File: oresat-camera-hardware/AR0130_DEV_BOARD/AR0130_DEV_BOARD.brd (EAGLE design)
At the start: 40 x 44 mm, 70 parts, among them J2 4-1734592-0, U10 SN74AVCB164245VR, U11 KC2520B27.0000C10E00, U12 TPS71818-33DRVT, U13 SN74AVCH8T245RHLR, U14 TPS71928-28DRVT, U15 TPS71928-28DRVT, U6 MCP9808T-E/MCDFN8_2X3MC-M, U7 MCP9808T-E/MCDFN8_2X3MC-M, U9 TCA9509DGKRDGK8-M

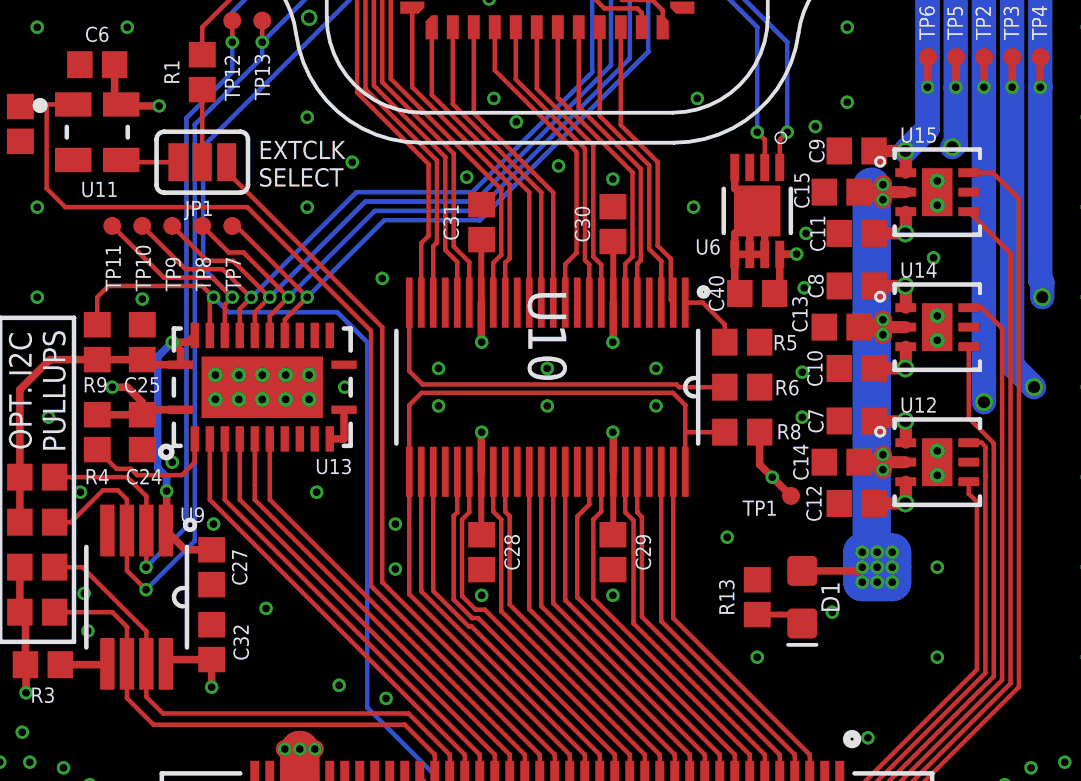
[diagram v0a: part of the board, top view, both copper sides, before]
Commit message: yada yada yada
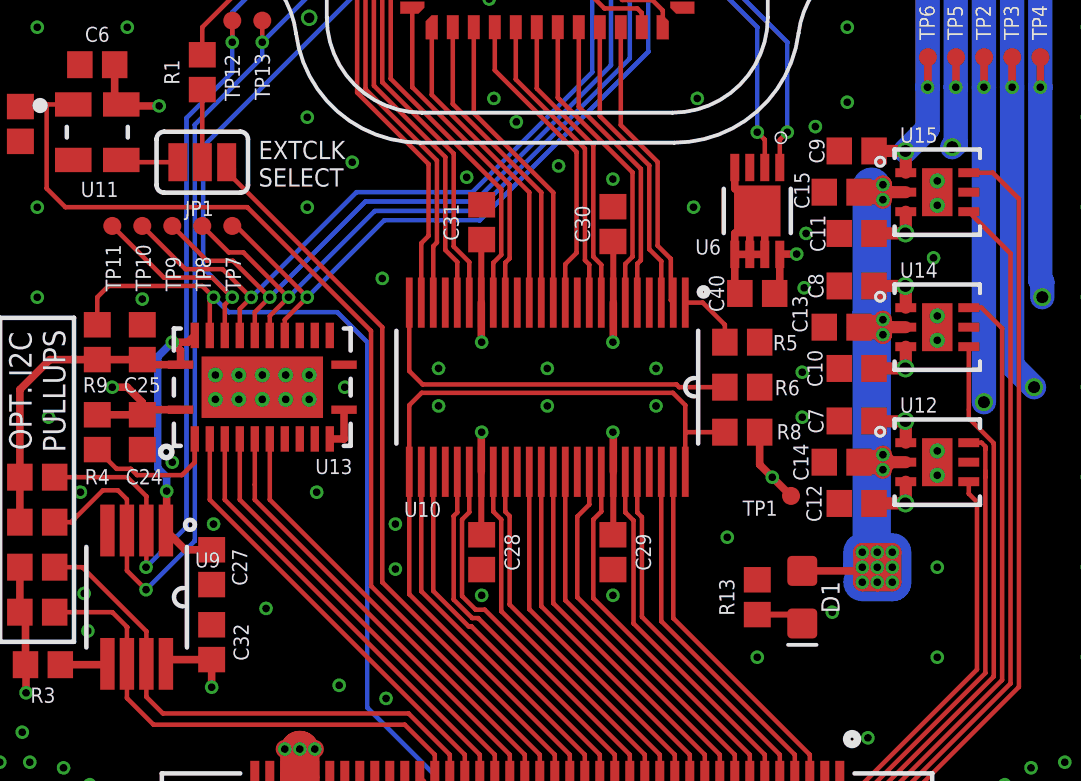
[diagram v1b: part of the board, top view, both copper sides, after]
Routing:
- net 5V: track 65.4 -> 70.4 mm
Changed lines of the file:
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@@
 <element name="U9" library="Oliver_Custom" package="DGK8-M" value="TCA9509DGKRDGK8-M" x="6.3125" y="11" smashed="yes" rot="R270">
 <attribute name="MANUFACTURER_PART_NUMBER" value="TCA9509DGKR" x="6.3125" y="11" size="1.778" layer="27" rot="R270" display="off"/>
-<attribute name="NAME" x="7.7574" y="13.4915" size="0.5" layer="25" font="vector" ratio="15" rot="SR0"/>
+<attribute name="NAME" x="8.2574" y="11.9915" size="0.5" layer="25" font="vector" ratio="15" rot="SR0"/>
 <attribute name="VENDOR" value="Texas Instruments" x="6.3125" y="11" size="1.778" layer="27" rot="R270" display="off"/>
 </element>
 <element name="U10" library="Oliver_Custom" package="DGV48" value="SN74AVCB164245VR" x="20" y="18" smashed="yes" rot="R270">
 <attribute name="MANUFACTURER_PART_NUMBER" value="SN74AVCB164245VR" x="20" y="18" size="1.778" layer="27" rot="R270" display="off"/>
-<attribute name="NAME" x="19.365" y="21.2766" size="1.27" layer="25" ratio="6" rot="SR270"/>
+<attribute name="NAME" x="15.2234" y="13.6775" size="0.5" layer="25" font="vector" ratio="15" rot="SR0"/>
 <attribute name="VENDOR" value="Texas Instruments" x="20" y="18" size="1.778" layer="27" rot="R270" display="off"/>
 </element>
@@
 <wire x1="30.5" y1="12" x2="31.5" y2="12" width="1.27" layer="16"/>
 <wire x1="30.5" y1="12" x2="30.5" y2="12.5" width="1.27" layer="16"/>
-<wire x1="30.5" y1="12.5" x2="30.5" y2="11.5" width="1.27" layer="16"/>
 <wire x1="31.5" y1="11.5" x2="31.5" y2="12.5" width="1.27" layer="16"/>
 <wire x1="30.5" y1="11.5" x2="31.5" y2="11.5" width="1.27" layer="16"/>
@@
 <wire x1="31.1875" y1="15.75" x2="31.1875" y2="15.5" width="0.508" layer="1"/>
 <wire x1="31.1875" y1="15.5" x2="31.1875" y2="15.25" width="0.508" layer="1"/>
-<wire x1="30.3925" y1="15.5" x2="31.1875" y2="15.5" width="0.6096" layer="1"/>
+<wire x1="30.3925" y1="15.5" x2="31.1875" y2="15.5" width="0.8128" layer="1"/>
 <wire x1="31.1875" y1="15.5" x2="31.95" y2="15.5" width="0.4064" layer="1"/>
 <via x="31.1875" y="19.75" extent="1-16" drill="0.254"/>
 <wire x1="31.1875" y1="19.75" x2="31.1875" y2="20.25" width="0.6096" layer="1"/>
-<wire x1="30.3925" y1="20" x2="30.9375" y2="20" width="0.6096" layer="1"/>
+<wire x1="30.3925" y1="20" x2="30.9375" y2="20" width="0.8128" layer="1"/>
 <wire x1="30.9375" y1="20" x2="31.1875" y2="19.75" width="0.6096" layer="1" curve="-90"/>
 <wire x1="31.95" y1="20" x2="31.4375" y2="20" width="0.4064" layer="1"/>
@@
 <via x="31.1875" y="24.25" extent="1-16" drill="0.254"/>
 <wire x1="31.1875" y1="24.75" x2="31.1875" y2="24.25" width="0.6096" layer="1"/>
-<wire x1="30.3925" y1="24.5" x2="30.9375" y2="24.5" width="0.6096" layer="1"/>
+<wire x1="30.3925" y1="24.5" x2="30.9375" y2="24.5" width="0.8128" layer="1"/>
 <wire x1="30.9375" y1="24.5" x2="31.1875" y2="24.75" width="0.6096" layer="1" curve="90"/>
 <wire x1="31.95" y1="24.5" x2="31.4375" y2="24.5" width="0.4064" layer="1"/>
@@
 <wire x1="31.5" y1="12.5" x2="31" y2="12.5" width="0.6096" layer="16"/>
 <wire x1="31" y1="12.5" x2="30.8125" y2="12.5" width="0.6096" layer="16"/>
+<wire x1="31" y1="12.5" x2="31" y2="11.5" width="0.6096" layer="1"/>
+<wire x1="30.5" y1="12.5" x2="30.5" y2="11.5" width="0.6096" layer="1"/>
+<wire x1="31" y1="12.5" x2="31" y2="11.5" width="0.6096" layer="1"/>
+<wire x1="31.5" y1="12.5" x2="31.5" y2="11.5" width="0.6096" layer="1"/>
+<wire x1="30.5" y1="12.5" x2="31.5" y2="12.5" width="0.6096" layer="1"/>
+<wire x1="30.5" y1="11.5" x2="31.5" y2="11.5" width="0.6096" layer="1"/>
 </signal>
 <signal name="GND">
